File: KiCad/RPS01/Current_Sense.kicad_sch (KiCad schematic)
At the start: 4 parts, among them U8 INA139QPWRQ1

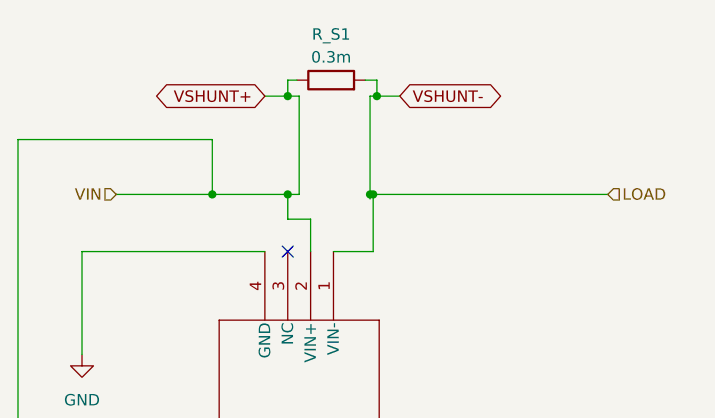
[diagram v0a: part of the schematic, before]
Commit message: Hotfix
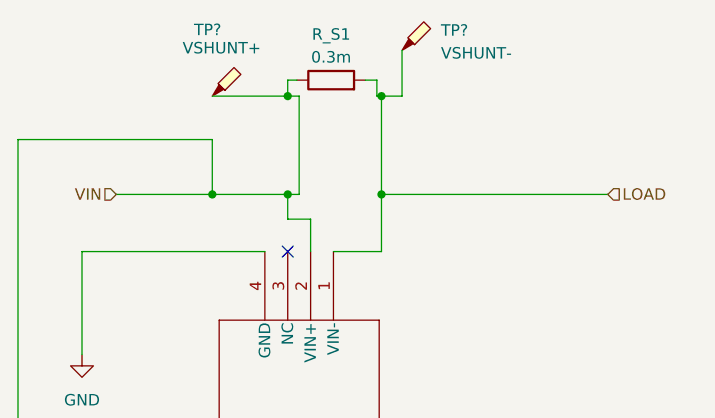
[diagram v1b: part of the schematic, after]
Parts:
- added TP?: VSHUNT-, Mechatronics TestP:CONN1_RCU-0C_TEC, symbol Connector:TestPoint_Probe
- added TP?: VSHUNT+, Mechatronics TestP:CONN1_RCU-0C_TEC, symbol Connector:TestPoint_Probe
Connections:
- net VSHUNT+ renamed VIN
- net VIN: now also TP?.1
- net VSHUNT- renamed LOAD
- net LOAD: now also TP?.1
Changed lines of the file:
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@@
   (junction (at 111.76 117.3986) (diameter 0) (color 0 0 0 0)
   )
-  (junction (at 114.046 24.638) (diameter 0) (color 0 0 0 0)
+  (junction (at 114.554 35.56) (diameter 0) (color 0 0 0 0)
   )
   (junction (at 104.14 24.638) (diameter 0) (color 0 0 0 0)
@@
   (junction (at 95.758 35.56) (diameter 0) (color 0 0 0 0)
   )
-  (junction (at 113.284 35.56) (diameter 0) (color 0 0 0 0)
-  )
-  (junction (at 113.6342 35.56) (diameter 0) (color 0 0 0 0)
-  )
   (junction (at 111.76 101.6158) (diameter 0) (color 0 0 0 0)
   )
+  (junction (at 114.554 24.638) (diameter 0) (color 0 0 0 0)
+  )
   (junction (at 121.92 100.5998) (diameter 0) (color 0 0 0 0)
   )
@@
     (stroke (width 0) (type default))
   )
+  (wire (pts (xy 116.84 24.638) (xy 114.554 24.638))
+    (stroke (width 0) (type default))
+  )
   (wire (pts (xy 114.046 22.86) (xy 114.046 24.638))
     (stroke (width 0) (type default))
@@
     (stroke (width 0) (type default))
   )
-  (wire (pts (xy 101.6 24.638) (xy 104.14 24.638))
-    (stroke (width 0) (type default))
-  )
   (wire (pts (xy 121.92 101.6158) (xy 121.92 105.41))
     (stroke (width 0) (type default))
@@
     (stroke (width 0) (type default))
   )
+  (wire (pts (xy 95.758 24.638) (xy 104.14 24.638))
+    (stroke (width 0) (type default))
+  )
   (wire (pts (xy 111.76 117.3986) (xy 111.76 119.38))
     (stroke (width 0) (type default))
   )
+  (wire (pts (xy 114.554 24.638) (xy 114.046 24.638))
+    (stroke (width 0) (type default))
+  )
   (wire (pts (xy 104.14 22.86) (xy 104.14 24.638))
     (stroke (width 0) (type default))
@@
     (stroke (width 0) (type default))
   )
-  (wire (pts (xy 111.76 101.6158) (xy 121.92 101.6158))
+  (wire (pts (xy 114.554 35.56) (xy 114.554 41.91))
     (stroke (width 0) (type default))
   )
-  (wire (pts (xy 113.284 24.638) (xy 114.046 24.638))
+  (wire (pts (xy 111.76 101.6158) (xy 121.92 101.6158))
     (stroke (width 0) (type default))
   )
@@
     (stroke (width 0) (type default))
   )
-  (wire (pts (xy 113.284 35.56) (xy 113.6342 35.56))
-    (stroke (width 0) (type default))
-  )
   (wire (pts (xy 112.776 22.86) (xy 114.046 22.86))
     (stroke (width 0) (type default))
@@
     (stroke (width 0) (type default))
   )
-  (wire (pts (xy 116.586 24.638) (xy 114.046 24.638))
-    (stroke (width 0) (type default))
-  )
-  (wire (pts (xy 113.6342 35.56) (xy 139.7 35.56))
-    (stroke (width 0) (type default))
-  )
   (wire (pts (xy 95.758 29.464) (xy 95.758 35.56))
     (stroke (width 0) (type default))
@@
     (stroke (width 0) (type default))
   )
-  (wire (pts (xy 113.6342 41.91) (xy 109.22 41.91))
+  (wire (pts (xy 114.554 41.91) (xy 109.22 41.91))
     (stroke (width 0) (type default))
   )
@@
     (stroke (width 0) (type default))
   )
-  (wire (pts (xy 113.6342 35.56) (xy 113.6342 41.91))
+  (wire (pts (xy 114.554 24.638) (xy 114.554 35.56))
     (stroke (width 0) (type default))
   )
-  (wire (pts (xy 113.284 36.068) (xy 113.284 35.56))
+  (wire (pts (xy 114.554 35.56) (xy 139.7 35.56))
     (stroke (width 0) (type default))
   )
@@
     (stroke (width 0) (type default))
   )
-  (wire (pts (xy 121.92 100.5998) (xy 136.144 100.5998))
+  (wire (pts (xy 116.84 19.558) (xy 116.84 24.638))
     (stroke (width 0) (type default))
   )
-  (wire (pts (xy 113.284 24.638) (xy 113.284 35.56))
+  (wire (pts (xy 121.92 100.5998) (xy 136.144 100.5998))
     (stroke (width 0) (type default))
   )
@@
     )
   )
-  (global_label "VSHUNT-" (shape bidirectional) (at 116.586 24.638 0) (fields_autoplaced)
-    (effects (font (size 1.27 1.27)) (justify left))
-    (property "Intersheetrefs" "${INTERSHEET_REFS}" (at 129.4327 24.638 0)
-      (effects (font (size 1.27 1.27)) (justify left) hide)
-    )
-  )
-  (global_label "VSHUNT+" (shape bidirectional) (at 101.6 24.638 180) (fields_autoplaced)
-    (effects (font (size 1.27 1.27)) (justify right))
-    (property "Intersheetrefs" "${INTERSHEET_REFS}" (at 88.7533 24.638 0)
-      (effects (font (size 1.27 1.27)) (justify right) hide)
-    )
-  )
   (global_label "CURRENT1" (shape bidirectional) (at 134.112 94.742 0) (fields_autoplaced)
     (effects (font (size 1.27 1.27)) (justify left))
@@
     (effects (font (size 1.27 1.27)) (justify right))
   )
+  (symbol (lib_id "Connector:TestPoint_Probe") (at 116.84 19.558 0) (unit 1)
+    (in_bom yes) (on_board yes) (dnp no) (fields_autoplaced)
+    (property "Reference" "TP?" (at 121.158 17.3355 0)
+      (effects (font (size 1.27 1.27)) (justify left))
+    )
+    (property "Value" "VSHUNT-" (at 121.158 19.8755 0)
+      (effects (font (size 1.27 1.27)) (justify left))
+    )
+    (property "Footprint" "Mechatronics TestP:CONN1_RCU-0C_TEC" (at 121.92 19.558 0)
+      (effects (font (size 1.27 1.27)) hide)
+    )
+    (property "Datasheet" "~" (at 121.92 19.558 0)
+      (effects (font (size 1.27 1.27)) hide)
+    )
+    (pin "1")
+    (instances
+      (project "rps01"
+        (path "/14930f15-c0a0-4b55-93e6-b112548415f6/577d3fc4-735f-4981-a3a1-4300f23b9ae6"
+          (reference "TP?") (unit 1)
+        )
+        (path "/14930f15-c0a0-4b55-93e6-b112548415f6/13e150ee-6c46-47a5-9c09-3749eb0dcbfe"
+          (reference "TP1") (unit 1)
+        )
+      )
+    )
+  )
   (symbol (lib_id "power:GND") (at 81.28 53.34 0) (unit 1)
     (in_bom yes) (on_board yes) (dnp no) (fields_autoplaced)
@@
         )
       )
+    )
+  )
+  (symbol (lib_id "Connector:TestPoint_Probe") (at 95.758 24.638 0) (unit 1)
+    (in_bom yes) (on_board yes) (dnp no)
+    (property "Reference" "TP?" (at 93.726 17.272 0)
+      (effects (font (size 1.27 1.27)) (justify left))
+    )
+    (property "Value" "VSHUNT+" (at 92.456 19.304 0)
+      (effects (font (size 1.27 1.27)) (justify left))
+    )
+    (property "Footprint" "Mechatronics TestP:CONN1_RCU-0C_TEC" (at 100.838 24.638 0)
+      (effects (font (size 1.27 1.27)) hide)
+    )
+    (property "Datasheet" "~" (at 100.838 24.638 0)
+      (effects (font (size 1.27 1.27)) hide)
+    )
+    (pin "1")
+    (instances
+      (project "rps01"
+        (path "/14930f15-c0a0-4b55-93e6-b112548415f6/577d3fc4-735f-4981-a3a1-4300f23b9ae6"
+          (reference "TP?") (unit 1)
+        )
+        (path "/14930f15-c0a0-4b55-93e6-b112548415f6/13e150ee-6c46-47a5-9c09-3749eb0dcbfe"
+          (reference "TP2") (unit 1)
+        )
+      )
